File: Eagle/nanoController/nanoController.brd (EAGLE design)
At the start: 36.9 x 47 mm, 9 parts

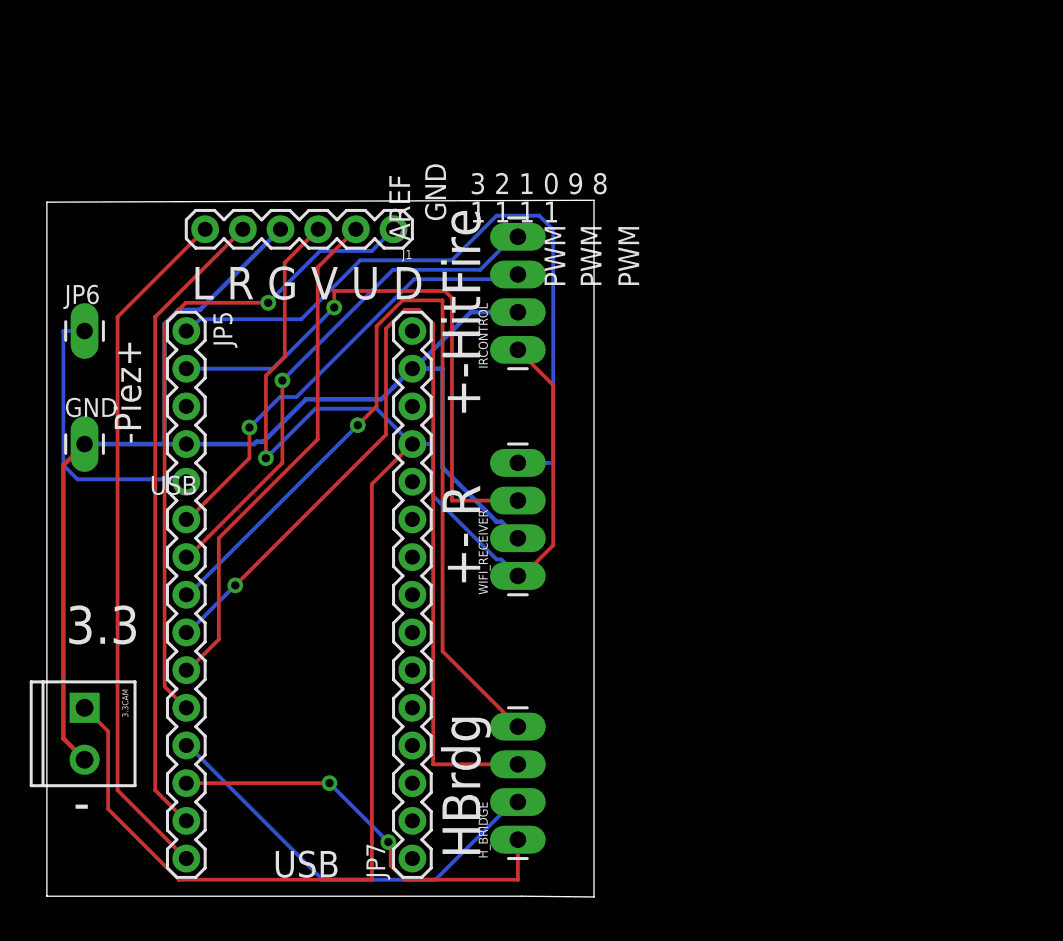
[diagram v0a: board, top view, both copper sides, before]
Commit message: webserver
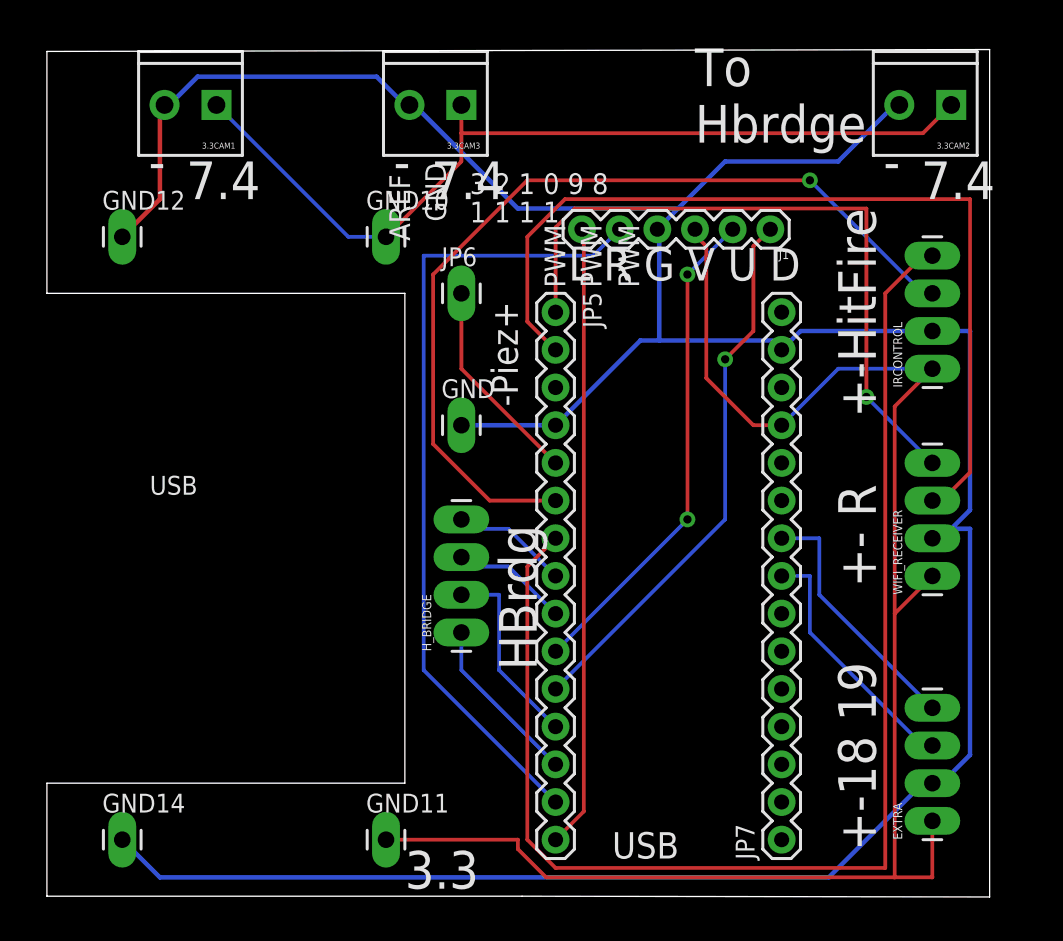
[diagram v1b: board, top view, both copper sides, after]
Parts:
- removed 3.3CAM: Power, SparkFun-Connectors:SCREWTERMINAL-3.5MM-2
- added 3.3CAM1, 3.3CAM2, 3.3CAM3: Power, SparkFun-Connectors:SCREWTERMINAL-3.5MM-2
- added EXTRA: (no value), SparkFun-Connectors:1X04_LONGPADS
- added GND10, GND11, GND12, GND14: (no value), SparkFun-Connectors:1X01_LONGPAD
- moved IRCONTROL 28.0 mm to (59.7, 35.6)
- moved WIFI_RECEIVER 27.9 mm to (59.7, 21.6)
- moved JP6 25.5 mm to (27.9, 40.6)
- moved GND 25.4 mm to (27.9, 31.8)
- moved J1 25.4 mm to (48.8, 45.0)
- moved JP5 24.9 mm to (34.3, 39.4)
- moved JP7 24.9 mm to (49.5, 3.81)
- moved H_BRIDGE 14.5 mm to (27.9, 17.8)
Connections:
- new net 7.4V: 3.3CAM1.1, 3.3CAM2.1, 3.3CAM3.1, GND10.1
- net D18: now also EXTRA.3
- net D19: now also EXTRA.4
- net GND: now also 3.3CAM1.2, 3.3CAM2.2, 3.3CAM3.2, EXTRA.2, GND12.1, GND14.1; no longer 3.3CAM.2
- net VCC: now also EXTRA.1, GND11.1; no longer 3.3CAM.1
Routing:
- net GND: track 89.7 -> 209.4 mm
- net 7.4V: track 0.00 -> 59.9 mm
- net D6: track 65.6 -> 7.93 mm, vias 1 -> 0
- net D4: track 34.5 -> 89.0 mm, vias 1 -> 0
- net D5: track 59.5 -> 7.93 mm, vias 1 -> 0
- net D3: track 30.4 -> 60.7 mm
- net D0: track 39.0 -> 61.1 mm, vias 1 -> 0
- net D19: track 0.00 -> 17.1 mm
- net D18: track 0.00 -> 17.1 mm
- net D10: track 28.6 -> 11.5 mm, vias 2 -> 0
- net D9: track 28.3 -> 13.0 mm
- net D11: track 43.2 -> 54.5 mm
- net VCC: track 117.1 -> 109.4 mm, vias 1 -> 0
- net D8: track 44.6 -> 37.0 mm
- net D2: track 19.2 -> 14.1 mm
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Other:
- board size 36.9 x 47 mm -> 63.6 x 57.1 mm
- board text added: "+-18 19"
- board text added: "7.4"
- board text added: "To Hbrdge"
